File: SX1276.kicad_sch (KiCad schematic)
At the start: 0 parts

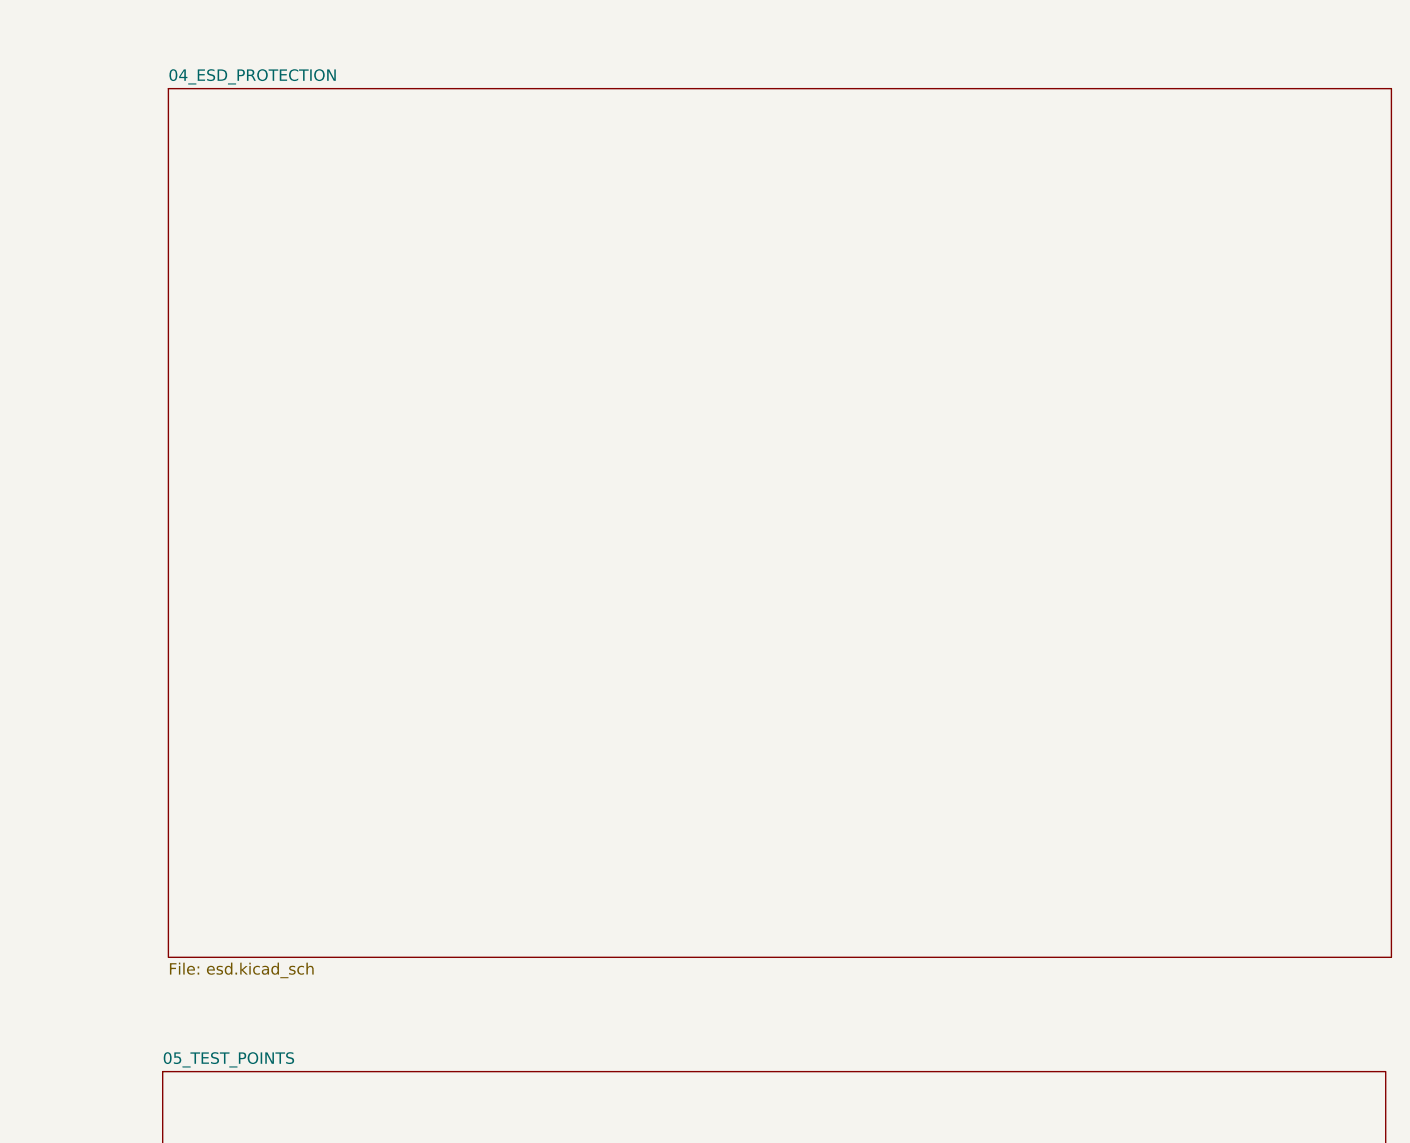
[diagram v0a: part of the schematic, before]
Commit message: connector update
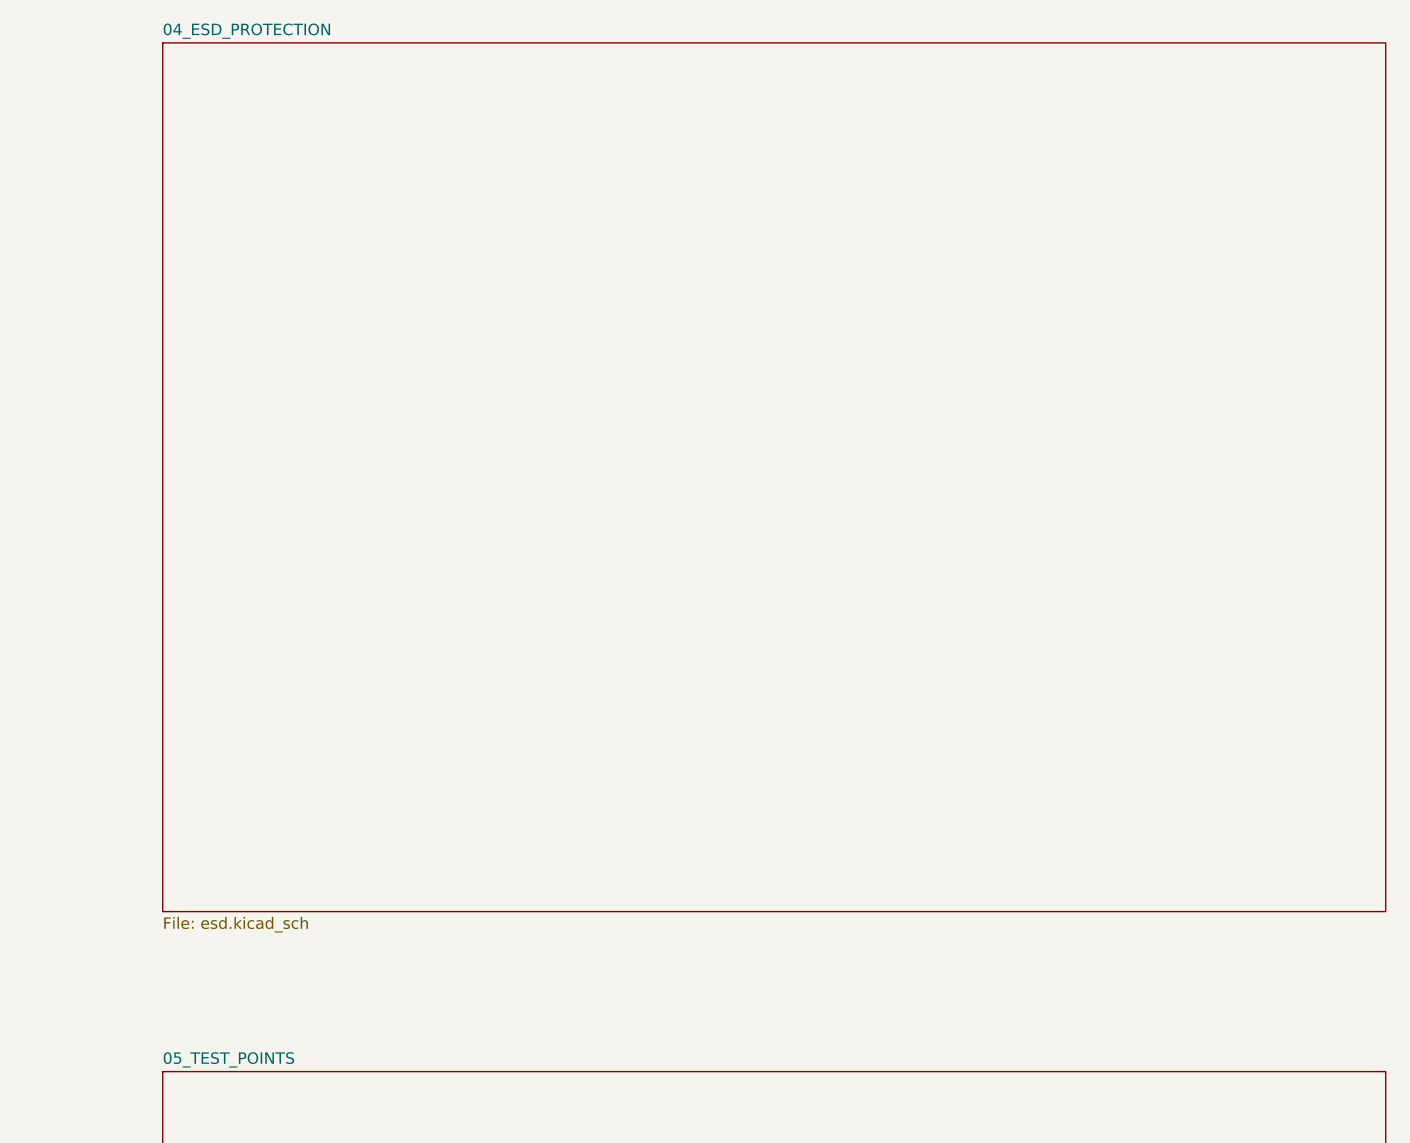
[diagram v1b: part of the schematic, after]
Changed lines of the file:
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@@
 	)
 	(sheet
-		(at 800.735 8.89)
+		(at 800.1 3.81)
 		(size 135.89 96.52)
 		(exclude_from_sim no)
@@
 		)
 		(property "Sheetname" "04_ESD_PROTECTION"
-			(at 800.735 8.1784 0)
+			(at 800.1 3.0984 0)
 			(effects
 				(font
@@
 		)
 		(property "Sheetfile" "esd.kicad_sch"
-			(at 800.735 105.9946 0)
+			(at 800.1 100.9146 0)
 			(effects
 				(font
